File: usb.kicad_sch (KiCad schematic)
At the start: 122 parts, among them J4 WE_632723300011_alt_symbol, U10 TUSB1046-DCI, U12 AP22615, U13 TPD4E05U06QDQARQ1, U14 TPD4E05U06QDQARQ1, U15 TPD4E05U06QDQARQ1, U16 TPD4E05U06QDQARQ1, U5 FT230XQ-R, U6 TPS65988, U7 W25Q80DVUXIE_TR, U8 NCP730BMT330TBG

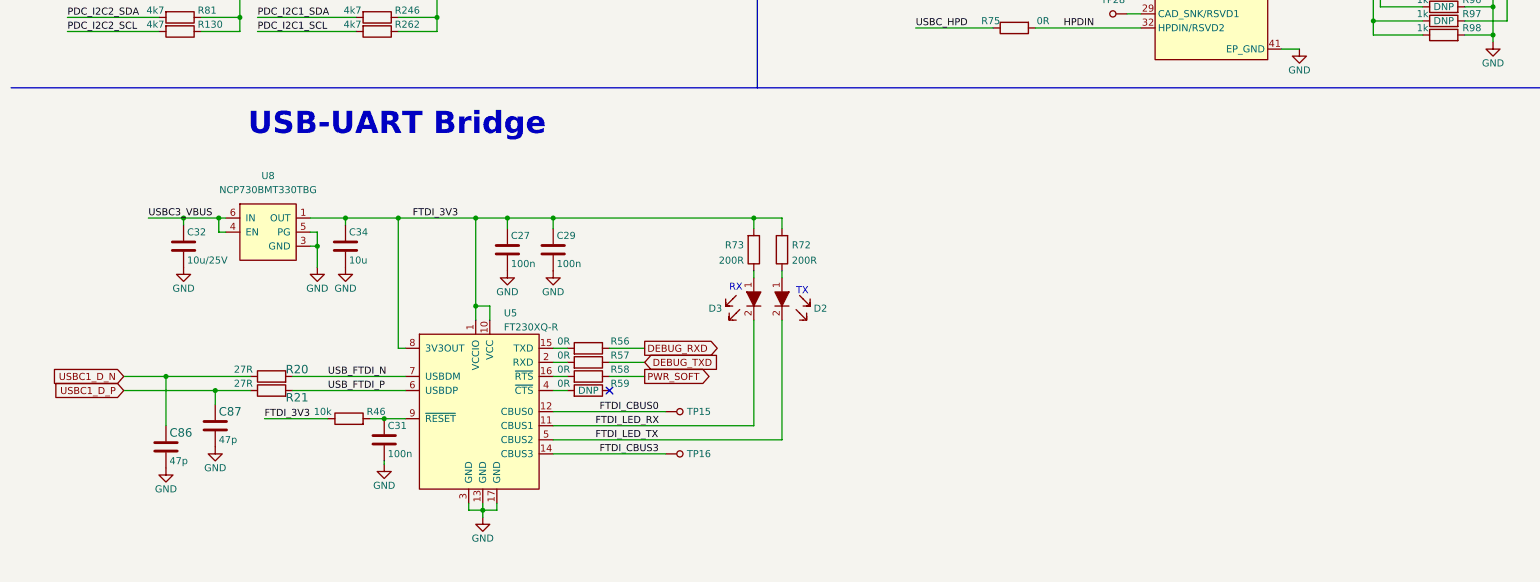
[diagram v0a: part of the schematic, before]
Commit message: 4G V1 Done
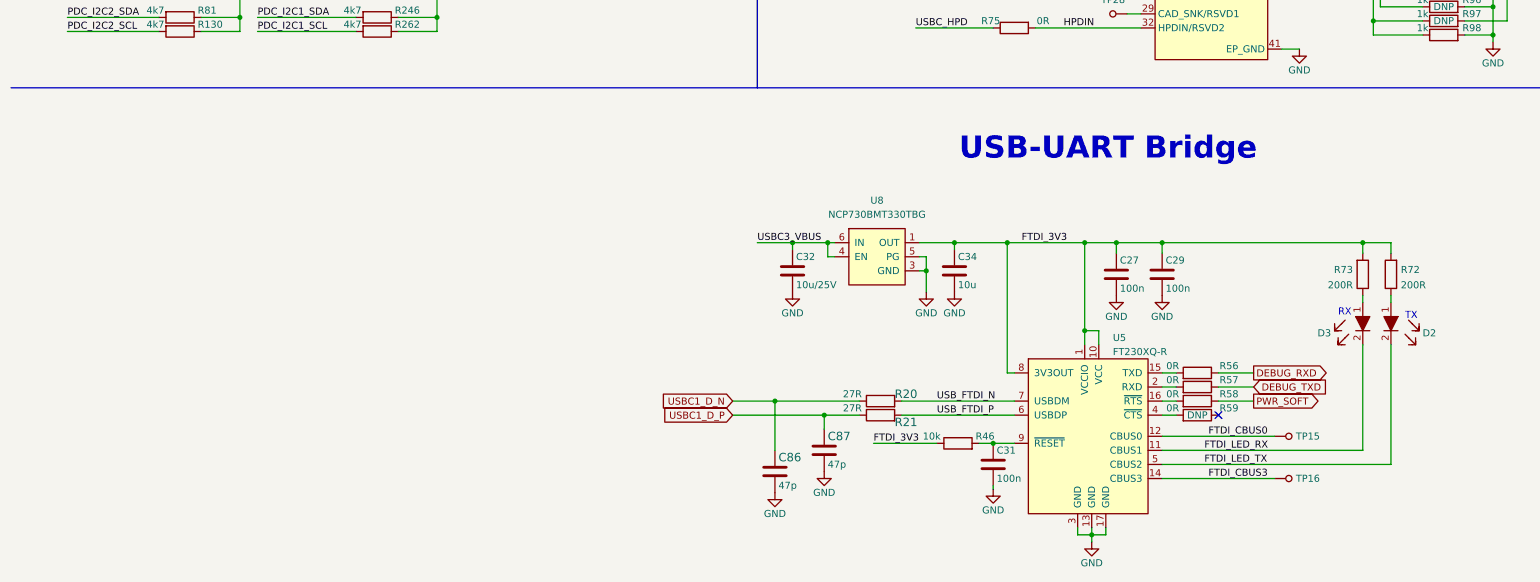
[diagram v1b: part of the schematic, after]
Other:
- moved on the sheet: C27, C29, C31, C32, C34, C86, C87, D2, D3, R20, R21, R46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
